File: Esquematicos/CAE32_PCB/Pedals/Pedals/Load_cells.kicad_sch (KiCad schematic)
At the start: 51 parts, among them J17 Conn_01x07_Female, J18 Conn_01x07_Female, J19 Conn_01x07_Female, Q1 MMBT3906, Q2 MMBT3906, Q3 MMBT3906, U5 HX711, U6 HX711, U7 HX711

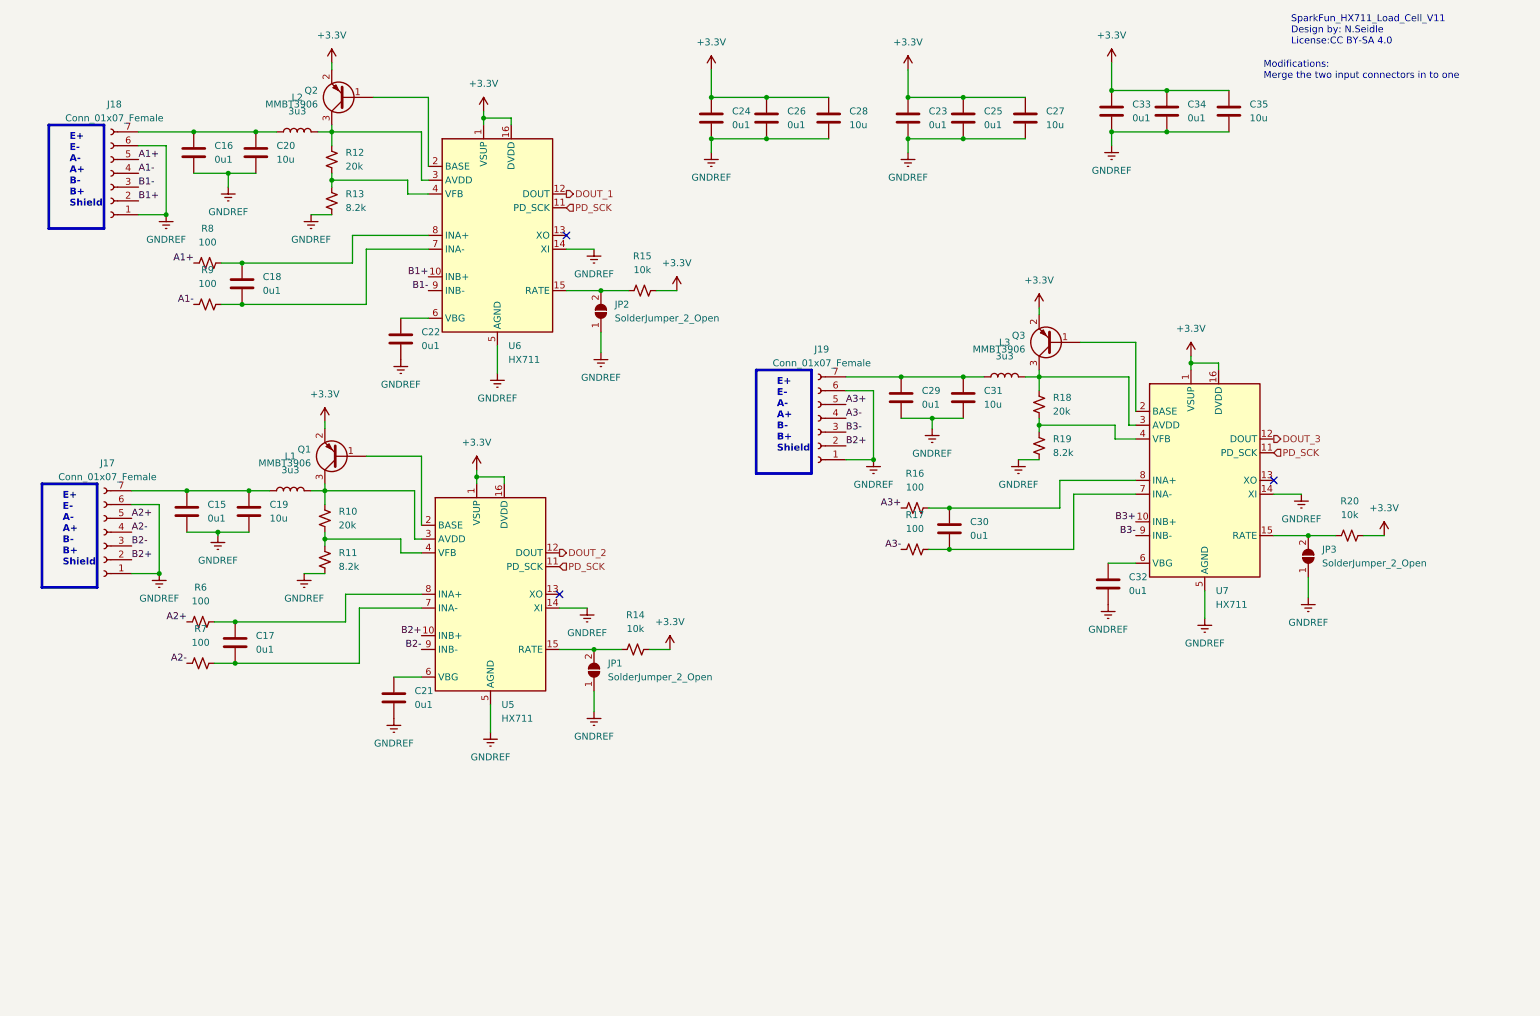
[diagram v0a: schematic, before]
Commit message: update: Componentes acomodados en la PCB
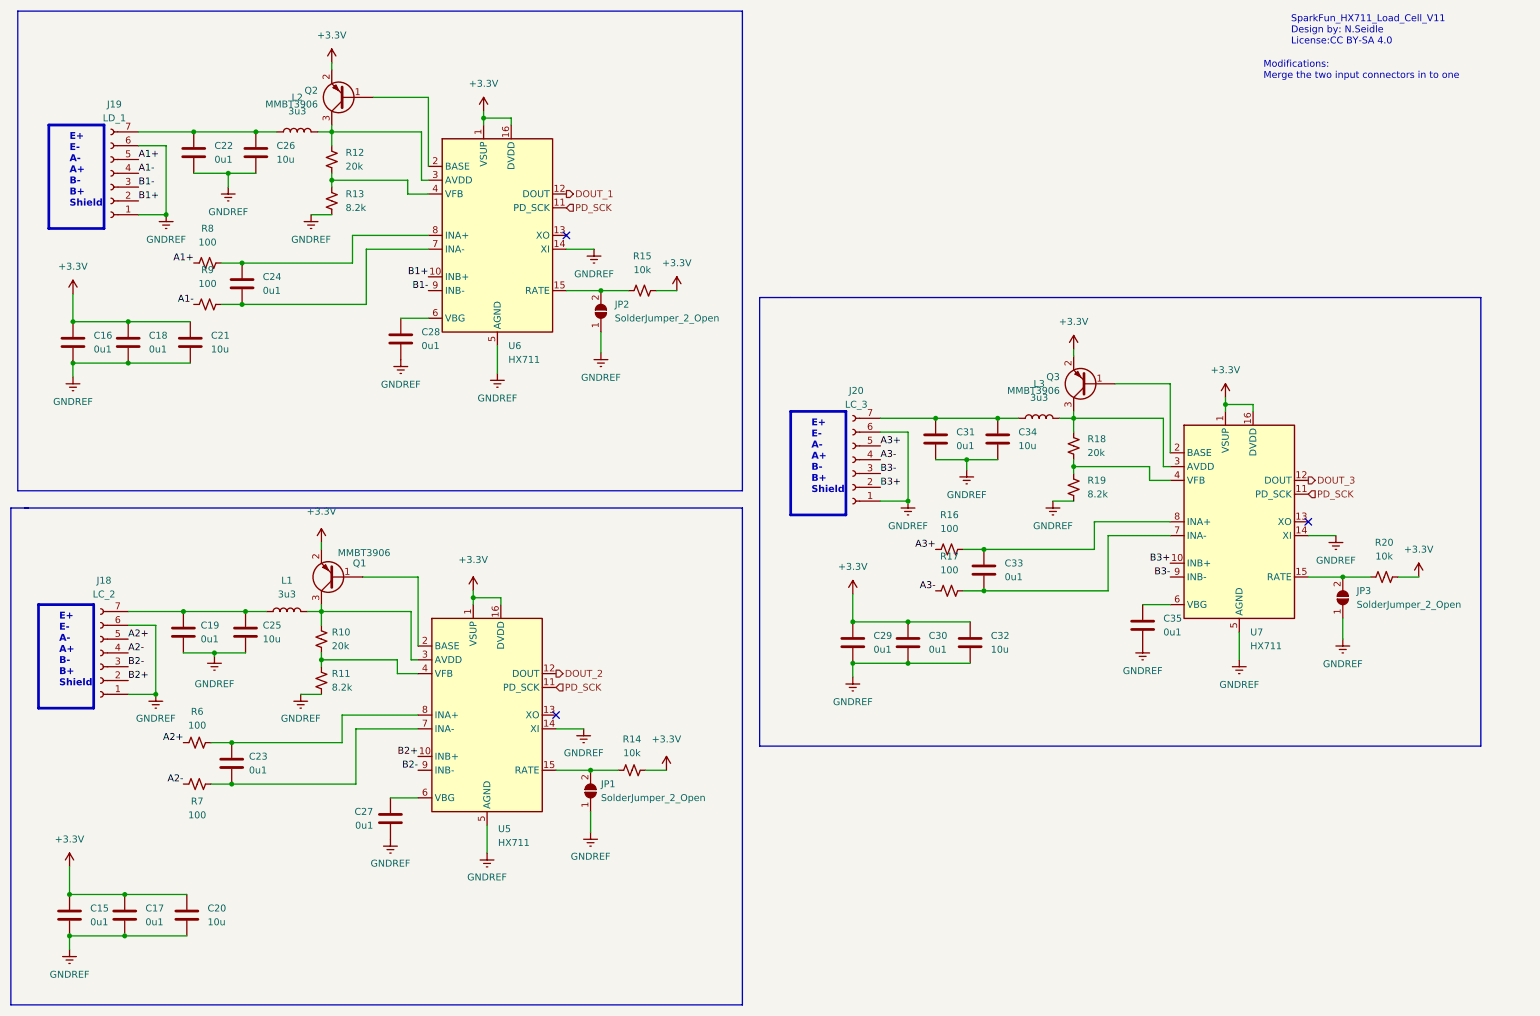
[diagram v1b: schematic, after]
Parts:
- J18: renamed from J17; value Conn_01x07_Female -> LC_2
- J19: renamed from J18; value Conn_01x07_Female -> LD_1
- J20: renamed from J19; value Conn_01x07_Female -> LC_3
- R10, R11, R12, R13, R14, R15, R16, R17, R18, R19, R20, R6, R7, R8, R9: footprint Resistor_SMD:R_0805_2012Metric_Pad1.20x1.40mm_HandSolder -> Resistor_SMD:R_0603_1608Metric_Pad0.98x0.95mm_HandSolder
- renumbered C23 to C15, C24 to C16, C25 to C17, C26 to C18, C15 to C19, C27 to C20, C28 to C21, C16 to C22, C17 to C23, C18 to C24, C19 to C25, C20 to C26, C21 to C27, C22 to C28, C33 to C29, C34 to C30, C29 to C31, C35 to C32, C30 to C33, C31 to C34, C32 to C35
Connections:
- net B2+: no longer J20.2 (Pin_2)
- net B3+: now also J20.2 (Pin_2)
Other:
- moved on the sheet: C15, C16, C17, C18, C19, C20, C21, C23, C25, C27, C29, C30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
